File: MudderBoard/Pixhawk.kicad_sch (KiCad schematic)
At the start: 23 parts, among them U1 TPS566242DRLR, U2 LP38691DTX-3.3/NOPB

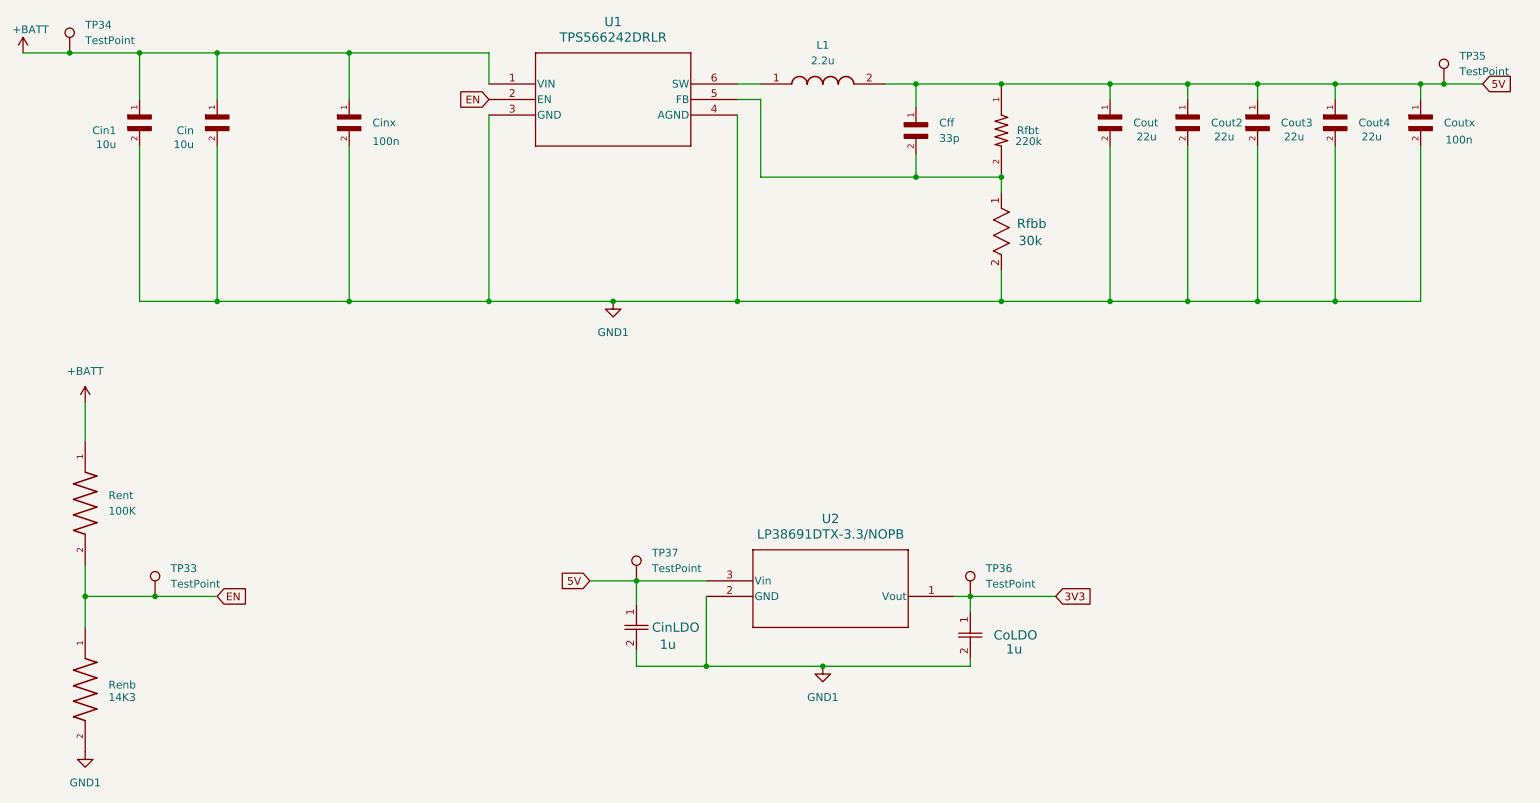
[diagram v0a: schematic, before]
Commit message: revert to eli changes
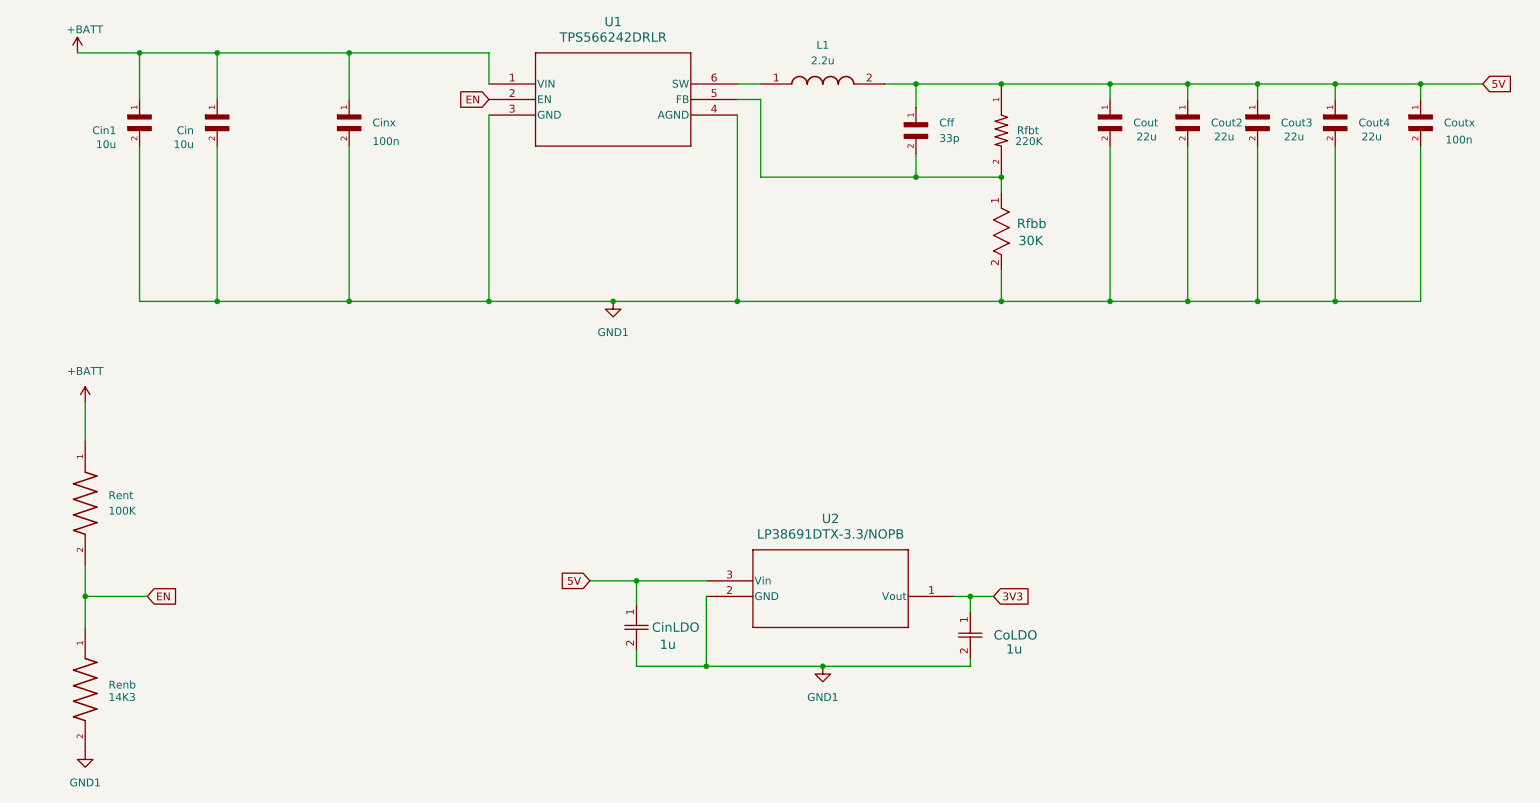
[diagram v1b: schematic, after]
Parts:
- removed TP33, TP34, TP35, TP36, TP37: TestPoint, TestPoint:TestPoint_Pad_D1.0mm, symbol Connector:TestPoint
- Rfbb: value 30k -> 30K
- Rfbt: value 220k -> 220K

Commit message: PixHawk Layout Updates
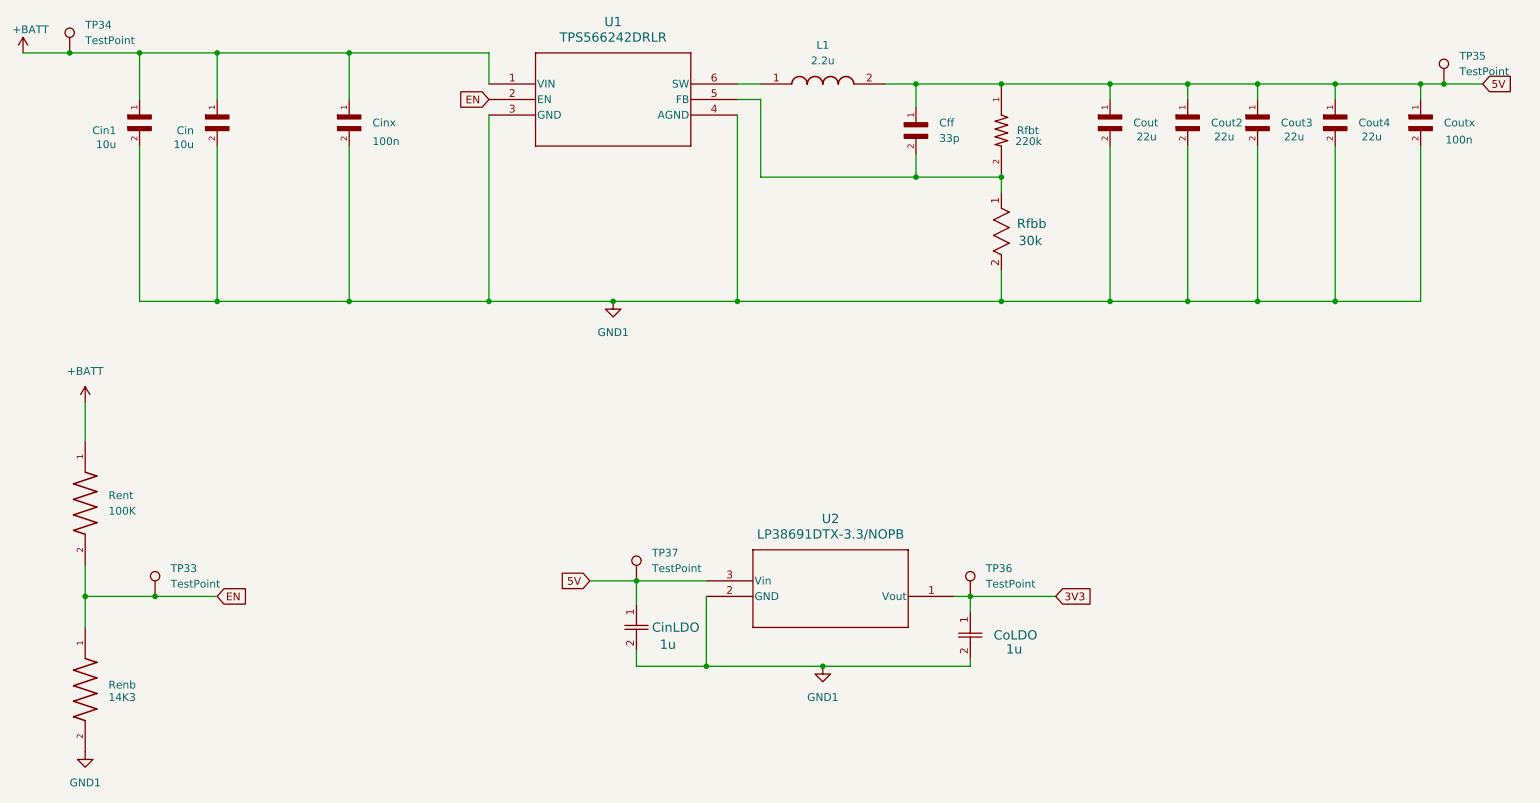
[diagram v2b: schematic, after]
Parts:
- added TP33, TP34, TP35, TP36, TP37: TestPoint, TestPoint:TestPoint_Pad_D1.0mm, symbol Connector:TestPoint
- Rfbb: value 30K -> 30k
- Rfbt: value 220K -> 220k
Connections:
- net +BATT: now also TP34.1
- net 3V3: now also TP36.1
- net 5V: now also TP35.1, TP37.1
- net EN: now also TP33.1
